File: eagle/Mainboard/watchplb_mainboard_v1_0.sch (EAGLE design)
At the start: 214 parts, among them IC1 LT1513, IC2 BM70BLES1FC2-0B03AA, IC3 LM1117DTX-ADJ-12V, IC4 AX5031, IC5 LM1117DTX-ADJ-10V, IC6 LM1117DTX-ADJ-3V3, J3 BNCPTH, Q1 8MHz / LFXTAL020423Reel, Q2 BC817-25SMD, Q3 DMN3023L-7, Q4 16MHz_LFXTAL051370Reel, Q5 CSD18534Q5A, Q6 CSD18534Q5A, Q7 DMN3023L-7, U1 MCP111-XXXXX/TO, U2 STM32L073RZ, U3 MCP2200-I/SS, U4 TPD3E001DRLR, U5 BQ7790504

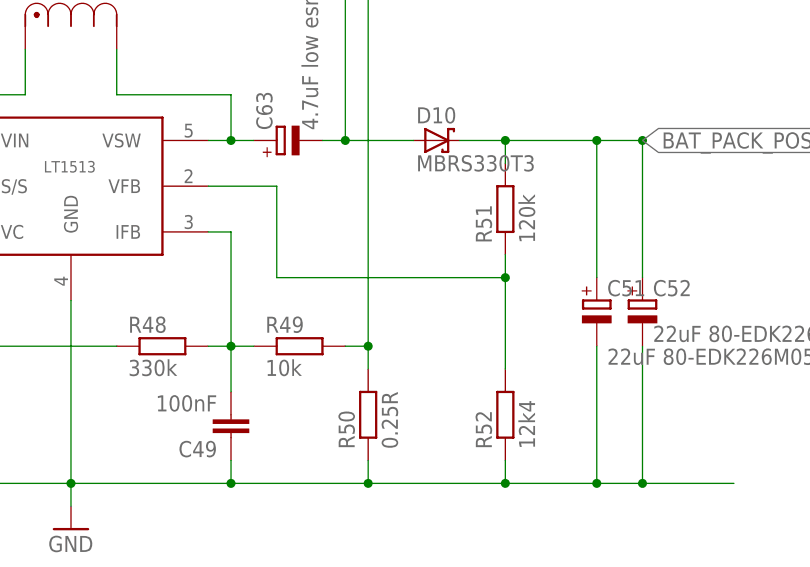
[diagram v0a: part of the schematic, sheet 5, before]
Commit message: Accumulated Changes over a few weeks
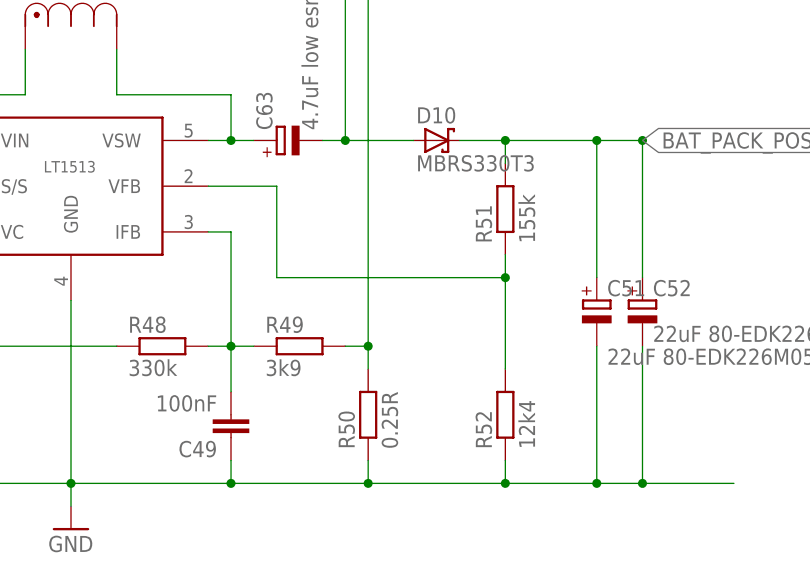
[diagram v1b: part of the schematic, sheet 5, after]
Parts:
- R49: value 10k -> 3k9
- R51: value 120k -> 155k
- R53: value 47k -> 5k1
- R54: value 5k1 -> 39k
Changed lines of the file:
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@@
 <part name="R48" library="resistor" deviceset="R-EU_" device="M0805" value="330k"/>
 <part name="C49" library="resistor" deviceset="C-EU" device="C0805K" value="100nF"/>
-<part name="R49" library="resistor" deviceset="R-EU_" device="M0805" value="10k"/>
+<part name="R49" library="resistor" deviceset="R-EU_" device="M0805" value="3k9"/>
 <part name="R50" library="resistor" deviceset="R-EU_" device="R2512" value="0.25R"/>
-<part name="R51" library="resistor" deviceset="R-EU_" device="M0805" value="120k"/>
+<part name="R51" library="resistor" deviceset="R-EU_" device="M0805" value="155k"/>
 <part name="R52" library="resistor" deviceset="R-EU_" device="M0805" value="12k4"/>
 <part name="C51" library="rcl" deviceset="CPOL-EU" device="E" value="22uF 80-EDK226M050A9GAA "/>
@@
 <part name="C53" library="rcl" deviceset="CPOL-EU" device="E" value="10uF  80-EDK106M025A9DAA  "/>
 <part name="C54" library="rcl" deviceset="CPOL-EU" device="E" value="100uF  647-GYA1E101MCQ1GS "/>
-<part name="R53" library="resistor" deviceset="R-EU_" device="M0805" value="47k"/>
-<part name="R54" library="resistor" deviceset="R-EU_" device="M0805" value="5k1"/>
+<part name="R53" library="resistor" deviceset="R-EU_" device="M0805" value="5k1"/>
+<part name="R54" library="resistor" deviceset="R-EU_" device="M0805" value="39k"/>
 <part name="P+2" library="supply1" deviceset="+12V" device=""/>
 <part name="C55" library="rcl" deviceset="CPOL-EU" device="E" value="NP"/>
